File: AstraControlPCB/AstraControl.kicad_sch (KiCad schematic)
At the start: 0 parts

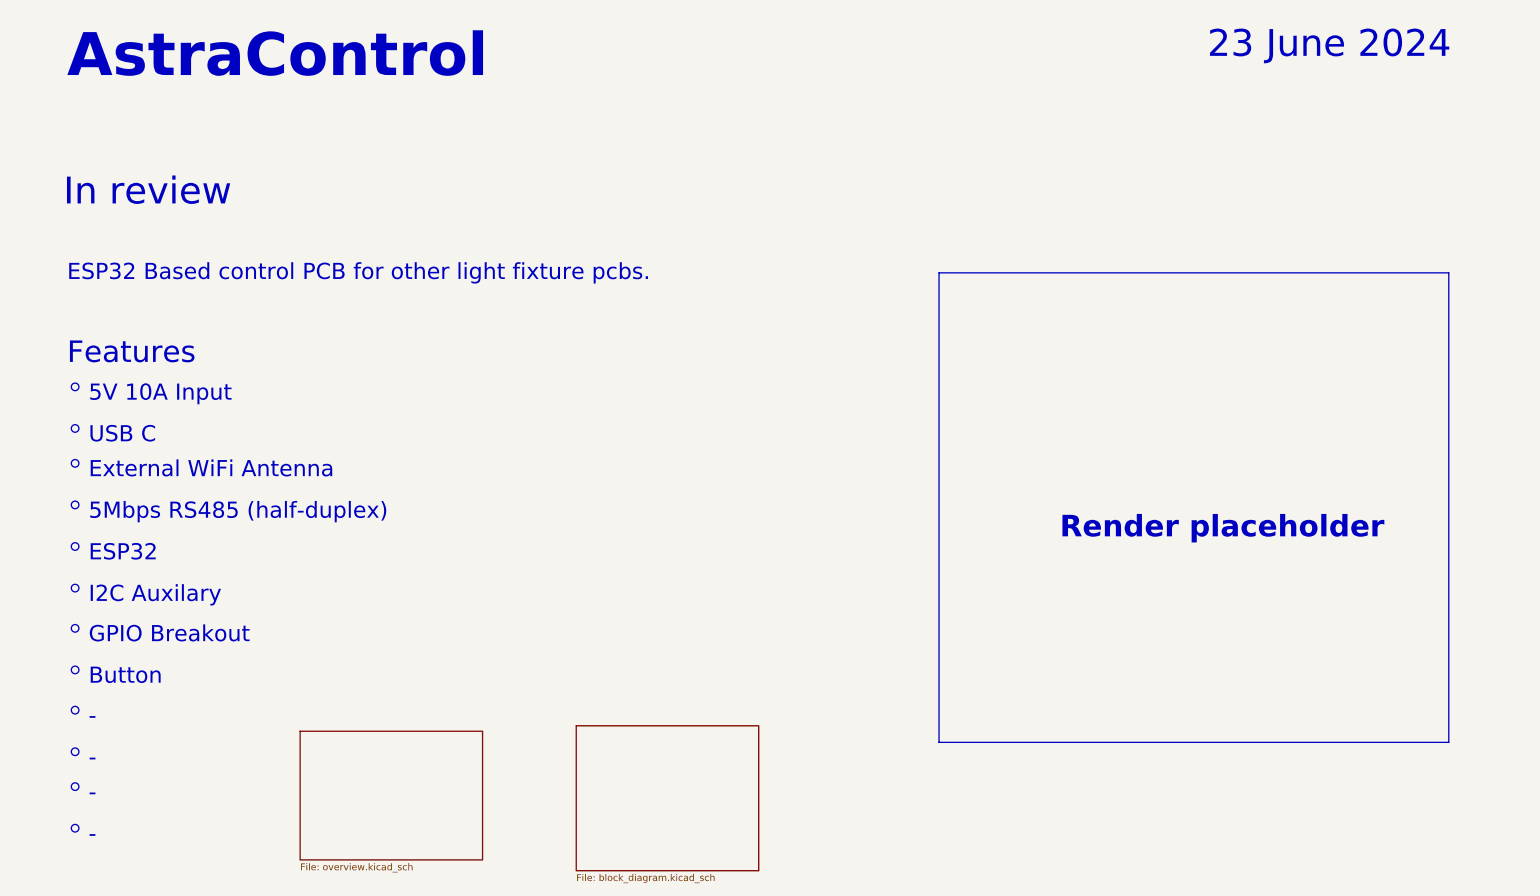
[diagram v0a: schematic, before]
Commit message: workflow
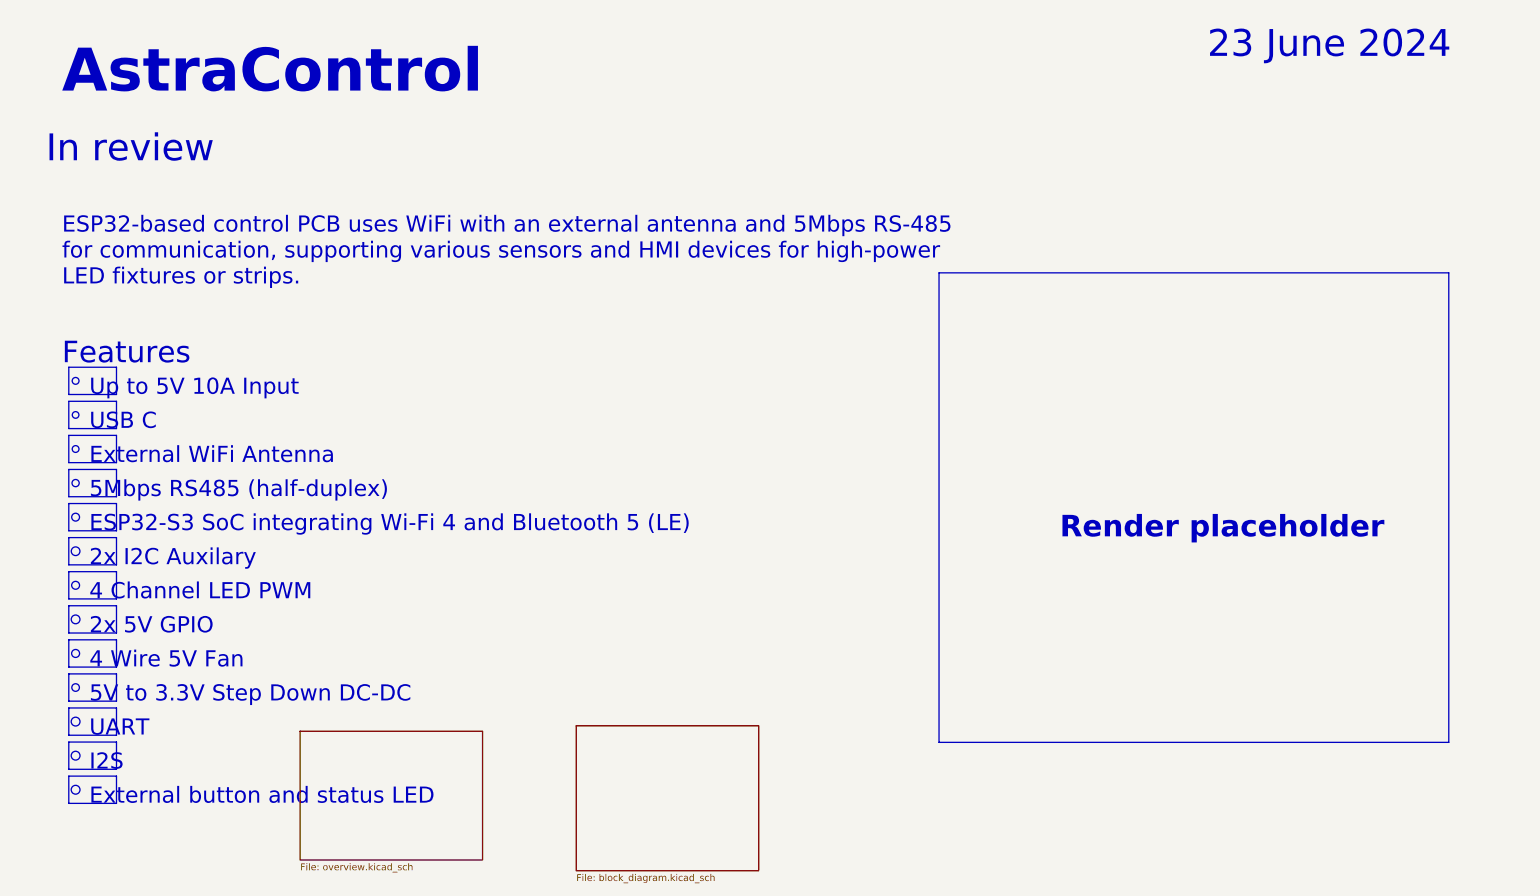
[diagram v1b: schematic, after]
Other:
- note added: "2x 5V GPIO"
- note added: "2x I2C Auxilary"
- note added: "4 Channel LED PWM"
- note added: "4 Wire 5V Fan"
- note added: "5V to 3.3V Step Down DC-DC"
- note added: "ESP32-S3 SoC integrating Wi-Fi 4 and Bluetooth 5 (LE)"
- note added: "ESP32-based control PCB uses WiFi with an external antenna and 5Mbps RS-485 for communication, supporting various sensors and HMI devices for high-power LED fixtures or strips."
- note added: "External button and status LED"
- note added: "I2S"
- note added: "UART"
- note added: "Up to 5V 10A Input"
- note removed: "-"
- note removed: "5V 10A Input"
- note removed: "Button"
- note removed: "ESP32"
- note removed: "ESP32 Based control PCB for other light fixture pcbs."
- note removed: "GPIO Breakout"
- note removed: "I2C Auxilary"
